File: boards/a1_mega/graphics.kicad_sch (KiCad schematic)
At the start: 16 parts, among them J5 Conn_01x02, J6 HDMI_A, U24 DISCO, U25 NAU8822, U35 74LVC06, X1 CXO_DIP14

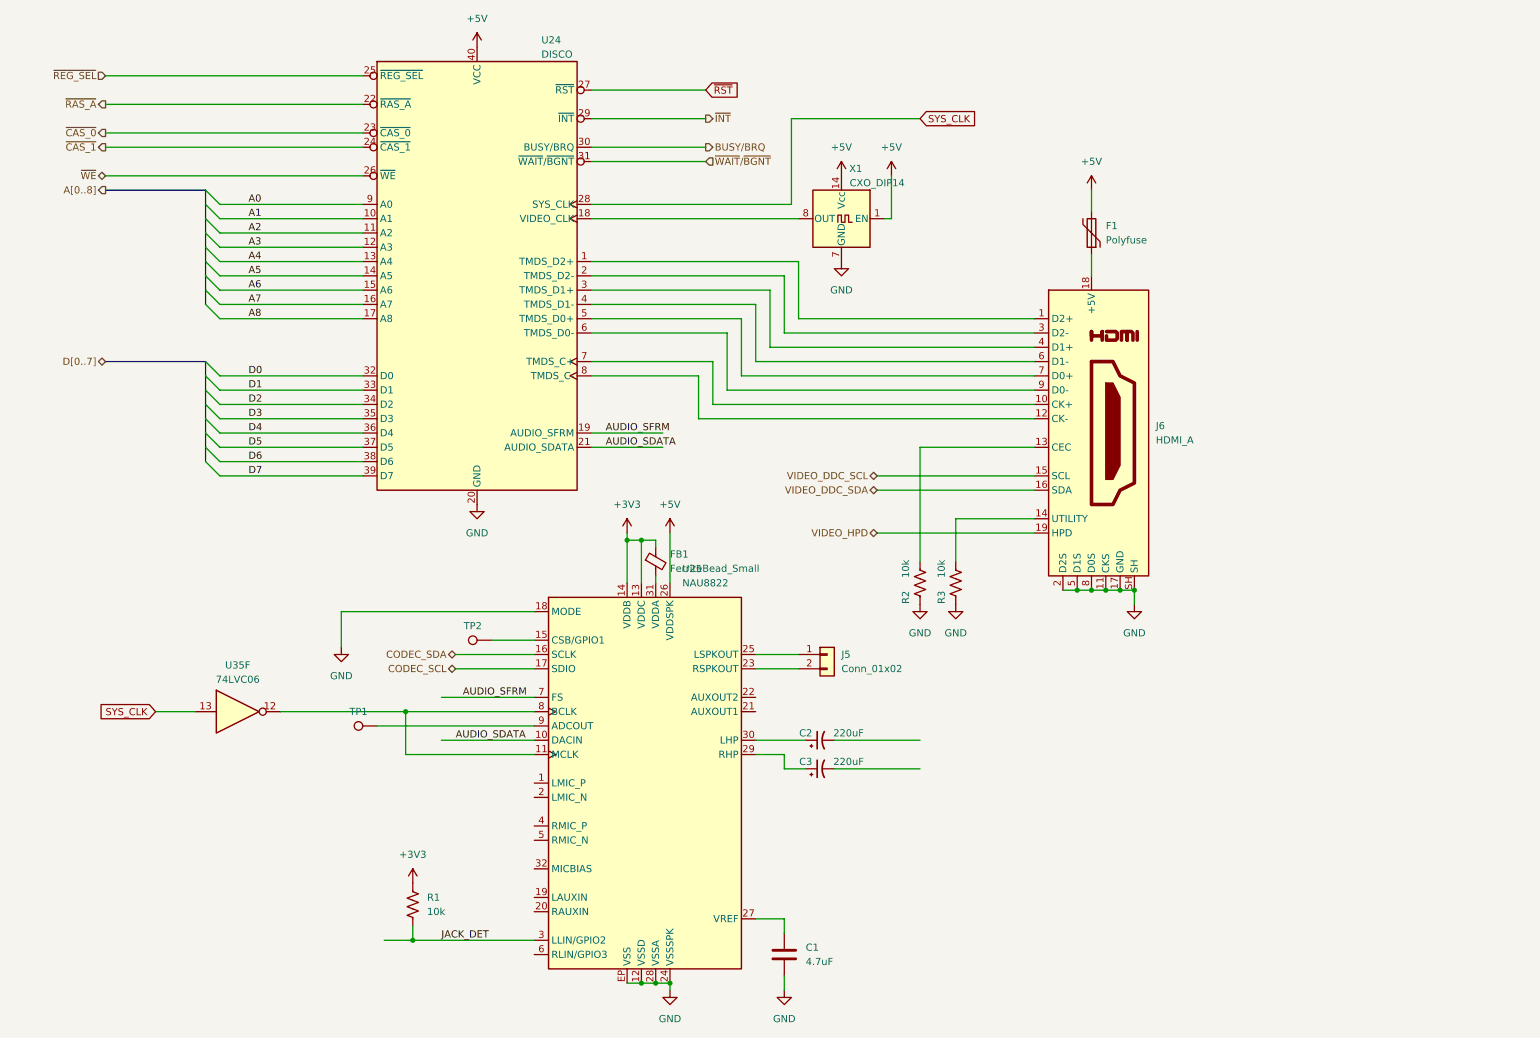
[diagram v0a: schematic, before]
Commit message: Extracted LAN chip, more progress towards full schematic.
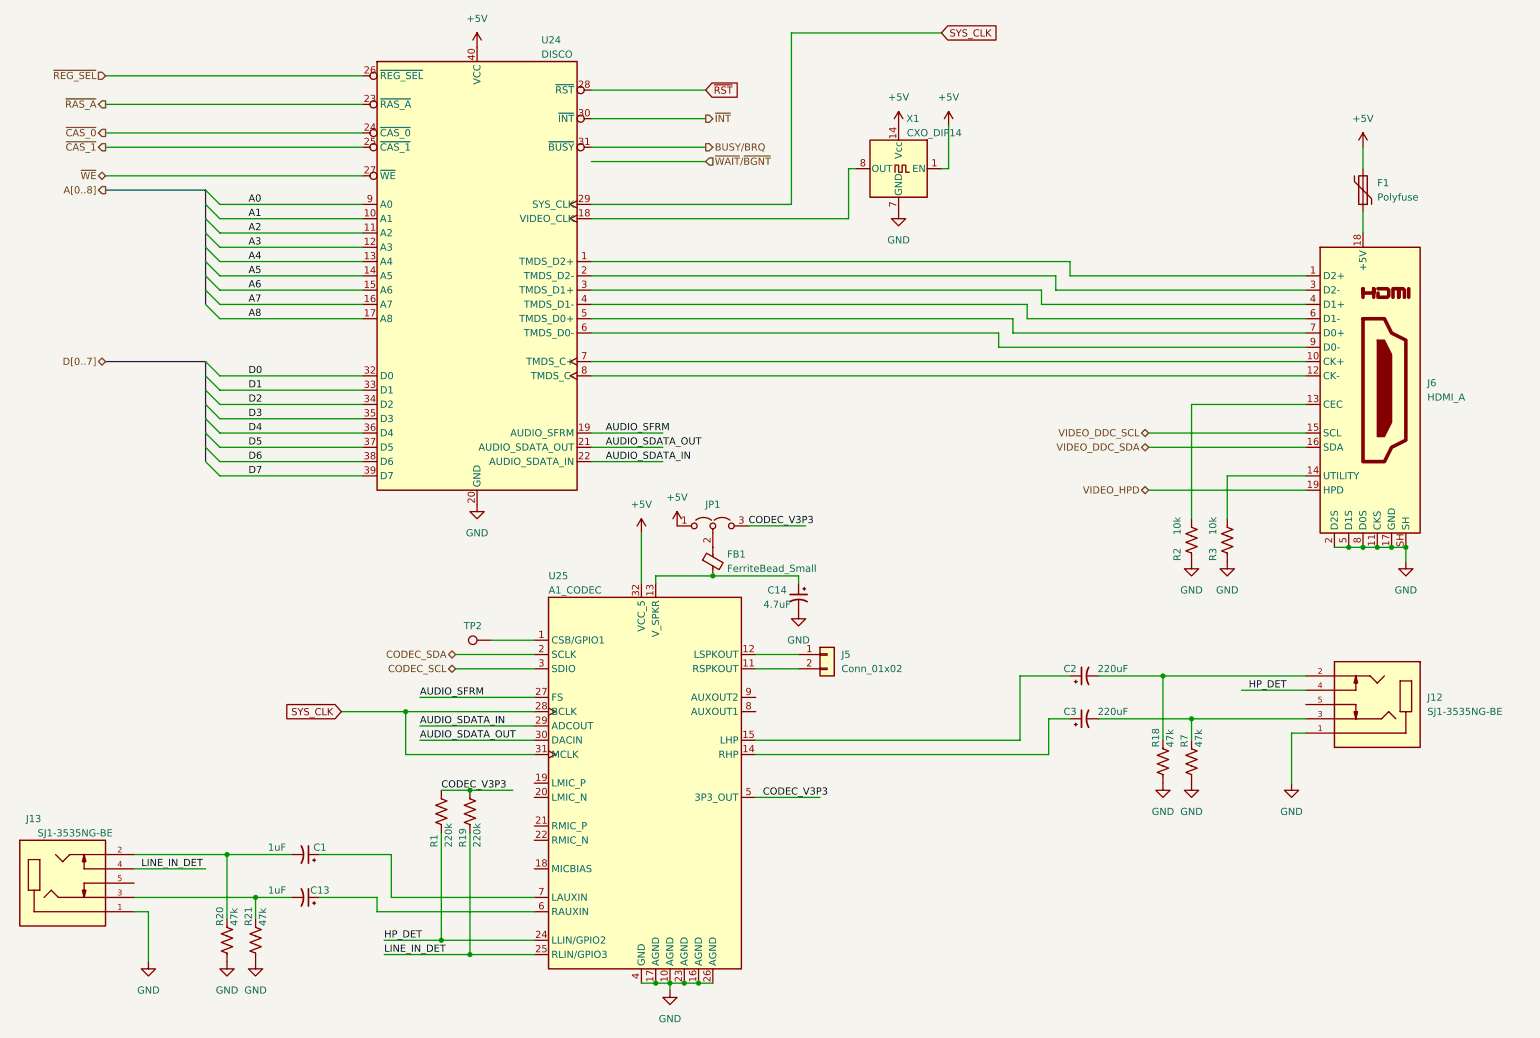
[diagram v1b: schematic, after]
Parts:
- removed C1: 4.7uF, Capacitor_THT:C_Rect_L9.0mm_W2.5mm_P7.50mm_MKT, symbol Device:C
- removed TP1: TestPoint_Alt, TestPoint:TestPoint_Plated_Hole_D2.0mm, symbol Connector:TestPoint
- removed U35: 74LVC06, Package_DIP:DIP-14_W7.62mm_LongPads, symbol 74xx:74LS06
- added C1, C13: 1uF, Capacitor_THT:CP_Radial_D4.0mm_P2.00mm, symbol Device:C_Polarized_Small_US
- added C14: 4.7uF, Capacitor_THT:CP_Radial_D4.0mm_P2.00mm, symbol Device:C_Polarized_Small_US
- added J12, J13: SJ1-3535NG-BE, anachron:CUI_SJ1-3535NG-BE, symbol anachron:SJ1-3535NG-BE
- added JP1: Jumper_3_Open, Connector_PinHeader_2.54mm:PinHeader_1x03_P2.54mm_Vertical, symbol Jumper:Jumper_3_Open
- added R18, R20, R21, R7: 47k, Resistor_THT:R_Axial_DIN0204_L3.6mm_D1.6mm_P5.08mm_Horizontal, symbol Device:R_US
- added R19: 220k, Resistor_THT:R_Axial_DIN0204_L3.6mm_D1.6mm_P5.08mm_Horizontal, symbol Device:R_US
- R1: value 10k -> 220k
- U25: value NAU8822 -> A1_CODEC; footprint Package_DFN_QFN:QFN-32-1EP_5x5mm_P0.5mm_EP3.1x3.1mm -> Package_DIP:DIP-32_W15.24mm_LongPads; symbol anachron:NAU8822 -> anachron:A1_CODEC
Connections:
- net +5V: now also U25.32 (VCC_5), JP1.1 (A); no longer U25.26 (VDDSPK)
- net AUDIO_SFRM: now also U25.27 (FS); no longer U25.7 (FS)
- net BUSY/BRQ: now also U24.31 (~{BUSY}); no longer U24.30 (BUSY/BRQ)
- net CODEC_SCL: now also U25.3 (SDIO); no longer U25.17 (SDIO)
- net CODEC_SDA: now also U25.2 (SCLK); no longer U25.16 (SCLK)
- net GND: now also U25.10 (AGND), U25.16 (AGND), U25.17 (AGND), U25.23 (AGND), U25.26 (AGND), U25.4 (GND), C14.2, J12.1, J13.1, R18.2, R20.2, R21.2, R7.2; no longer U25.12 (VSSD), U25.18 (MODE), U25.24 (VSSSPK), U25.28 (VSSA), U25.EP (VSS)
- net SYS_CLK: now also U24.29 (SYS_CLK), U25.28 (BCLK), U25.31 (MCLK); no longer U24.28 (SYS_CLK)
- net ~{CAS_0}: now also U24.24 (~{CAS_0}); no longer U24.23 (~{CAS_0})
- net ~{CAS_1}: now also U24.25 (~{CAS_1}); no longer U24.24 (~{CAS_1})
- net ~{INT}: now also U24.30 (~{INT}); no longer U24.29 (~{INT})
- net ~{RAS_A}: now also U24.23 (~{RAS_A}); no longer U24.22 (~{RAS_A})
- net ~{REG_SEL}: now also U24.26 (~{REG_SEL}); no longer U24.25 (~{REG_SEL})
- net ~{RST}: now also U24.28 (~{RST}); no longer U24.27 (~{RST})
- net ~{WAIT}/~{BGNT}: no longer U24.31 (~{WAIT}/~{BGNT})
- net ~{WE}: now also U24.27 (~{WE}); no longer U24.26 (~{WE})
- net at C2.1: now also U25.15 (LHP); no longer U25.30 (LHP)
- net at C2.2: now also J12.2, R18.1
- net at U25.1 (CSB/GPIO1): now also TP2.1
- net at U25.11 (RSPKOUT): now also J5.2 (Pin_2); no longer U25.8 (BCLK)
- net at J5.1 (Pin_1): now also U25.12 (LSPKOUT); no longer U25.25 (LSPKOUT)
- net at C3.1: now also U25.14 (RHP); no longer U25.29 (RHP)
- net at FB1.2: now also U25.13 (V_SPKR), C14.1; no longer U25.31 (VDDA)
- net CODEC_V3P3: now reaches U25.5 (3P3_OUT)
- net CODEC_V3P3: now also R1.1, JP1.3 (B), R19.1
- net at U25.6 (RAUXIN): now also C13.1
- net at C3.2: now also J12.3, R7.1
- removed net +3V3: FB1.1, R1.1, U25.13 (VDDC), U25.14 (VDDB)
- net AUDIO_SDATA renamed AUDIO_SDATA_OUT
- net AUDIO_SDATA_OUT: now also U25.30 (DACIN); no longer U25.10 (DACIN)
- net JACK_DET renamed HP_DET
- net HP_DET: now also U25.24 (LLIN/GPIO2), J12.4; no longer U25.3 (LLIN/GPIO2)
- new net: C13.2, J13.3, R21.1
- new net: C1.1, U25.7 (LAUXIN)
- new net: C1.2, J13.2, R20.1
- new net: FB1.1, JP1.2 (C)
- new net AUDIO_SDATA_IN: U24.22 (AUDIO_SDATA_IN), U25.29 (ADCOUT)
- new net LINE_IN_DET: J13.4, R19.2, U25.25 (RLIN/GPIO3)
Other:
- moved on the sheet: C2, C3, F1, FB1, J6, R1, R2, R3, X1
